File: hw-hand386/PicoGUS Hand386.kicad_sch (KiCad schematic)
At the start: 37 parts, among them J1 AudioJack3, J3 Bus_ISA_8bit, J5 AudioJack3, J6 UART_TX, U1 Pico, U2 SN74CB3T3245, U3 SN74CB3T3257, U4 SN74CB3T3257, U5 74AHC14, U6 74LVC00, U7 74LVC1G00, U8 APS6404L-3SQN-SN, U9 74LVC1G06

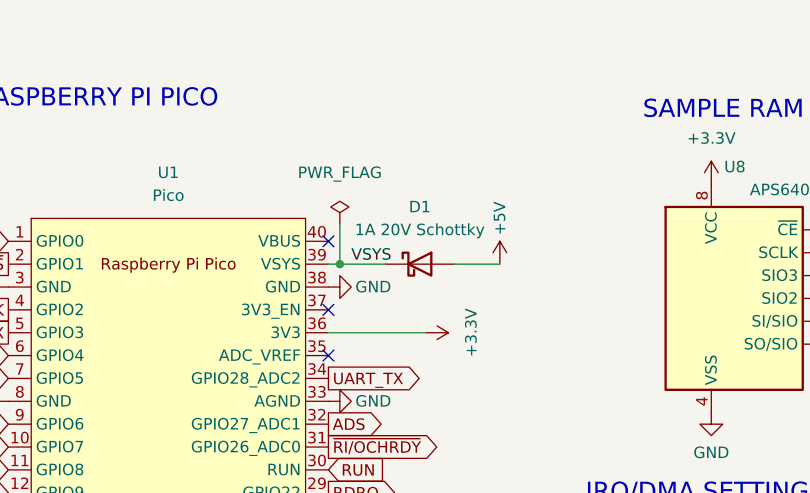
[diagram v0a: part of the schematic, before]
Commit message: v1.3 of Femto edition submitted to JLCPCB 2022-09-26
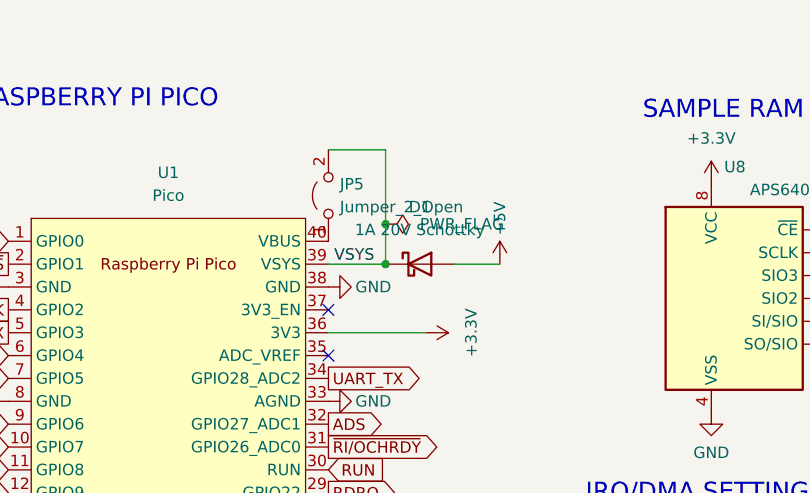
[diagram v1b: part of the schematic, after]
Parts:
- added JP5: Jumper_2_Open, Connector_PinHeader_2.54mm:PinHeader_1x02_P2.54mm_Vertical, symbol Jumper:Jumper_2_Open
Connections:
- net VSYS: now also JP5.2 (B)
- net at U1.40 (VBUS): now also JP5.1 (A)
- no-connect marks 6 -> 5
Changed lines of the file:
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@@
   (junction (at 62.865 182.88) (diameter 0) (color 0 0 0 0)
   )
+  (junction (at 133.35 40.005) (diameter 0) (color 0 0 0 0)
+  )
   (junction (at 217.805 160.655) (diameter 0) (color 0 0 0 0)
   )
@@
   (junction (at 89.535 166.37) (diameter 0) (color 0 0 0 0)
   )
-  (junction (at 128.27 40.005) (diameter 0) (color 0 0 0 0)
-  )
   (junction (at 233.68 153.035) (diameter 0) (color 0 0 0 0)
   )
@@
   )
   (junction (at 47.625 190.5) (diameter 0) (color 0 0 0 0)
+  )
+  (junction (at 133.35 35.56) (diameter 0) (color 0 0 0 0)
   )
   (junction (at 67.945 190.5) (diameter 0) (color 0 0 0 0)
@@
   (no_connect (at 145.415 121.285))
   (no_connect (at 127 50.165))
-  (no_connect (at 127 37.465))
   (no_connect (at 127 45.085))
   (no_connect (at 145.415 136.525))
@@
     (stroke (width 0) (type default))
   )
-  (wire (pts (xy 128.27 40.005) (xy 127 40.005))
+  (wire (pts (xy 127 40.005) (xy 133.35 40.005))
     (stroke (width 0) (type default))
   )
@@
     (stroke (width 0) (type default))
   )
-  (wire (pts (xy 128.27 35.56) (xy 128.27 40.005))
+  (wire (pts (xy 133.35 27.305) (xy 133.35 35.56))
     (stroke (width 0) (type default))
   )
@@
     (stroke (width 0) (type default))
   )
+  (wire (pts (xy 133.35 27.305) (xy 127 27.305))
+    (stroke (width 0) (type default))
+  )
   (wire (pts (xy 175.26 88.265) (xy 175.26 93.345))
     (stroke (width 0) (type default))
@@
     (stroke (width 0) (type default))
   )
-  (wire (pts (xy 133.35 40.005) (xy 128.27 40.005))
-    (stroke (width 0) (type default))
-  )
   (wire (pts (xy 21.59 100.33) (xy 28.575 100.33))
     (stroke (width 0) (type default))
@@
   )
   (wire (pts (xy 180.34 129.54) (xy 189.23 129.54))
+    (stroke (width 0) (type default))
+  )
+  (wire (pts (xy 133.35 35.56) (xy 133.35 40.005))
     (stroke (width 0) (type default))
   )
@@
     (effects (font (size 2 2)) (justify left bottom))
   )
-  (label "VSYS" (at 129.54 40.005 0) (fields_autoplaced)
+  (label "VSYS" (at 127.635 40.005 0) (fields_autoplaced)
     (effects (font (size 1.27 1.27)) (justify left bottom))
   )
@@
     )
   )
+  (symbol (lib_id "Jumper:Jumper_2_Open") (at 127 32.385 90) (unit 1)
+    (in_bom yes) (on_board yes) (dnp no)
+    (property "Reference" "JP5" (at 128.27 31.115 90)
+      (effects (font (size 1.27 1.27)) (justify right))
+    )
+    (property "Value" "Jumper_2_Open" (at 128.27 33.655 90)
+      (effects (font (size 1.27 1.27)) (justify right))
+    )
+    (property "Footprint" "Connector_PinHeader_2.54mm:PinHeader_1x02_P2.54mm_Vertical" (at 127 32.385 0)
+      (effects (font (size 1.27 1.27)) hide)
+    )
+    (property "Datasheet" "~" (at 127 32.385 0)
+      (effects (font (size 1.27 1.27)) hide)
+    )
+    (pin "1")
+    (pin "2")
+    (instances
+      (project "PicoGUS Hand386"
+        (path "/8fb4b197-630e-4faa-9892-8ecaeb71c13b"
+          (reference "JP5") (unit 1)
+        )
+      )
+    )
+  )
   (symbol (lib_id "Device:D_Schottky") (at 137.16 40.005 0) (unit 1)
     (in_bom yes) (on_board yes) (dnp no)
@@
     )
   )
-  (symbol (lib_id "power:PWR_FLAG") (at 128.27 35.56 0) (unit 1)
+  (symbol (lib_id "power:PWR_FLAG") (at 133.35 35.56 270) (unit 1)
     (in_bom yes) (on_board yes) (dnp no) (fields_autoplaced)
-    (property "Reference" "#FLG0101" (at 128.27 33.655 0)
-      (effects (font (size 1.27 1.27)) hide)
-    )
-    (property "Value" "PWR_FLAG" (at 128.27 29.845 0)
-      (effects (font (size 1.27 1.27)))
-    )
-    (property "Footprint" "" (at 128.27 35.56 0)
-      (effects (font (size 1.27 1.27)) hide)
-    )
-    (property "Datasheet" "~" (at 128.27 35.56 0)
-      (effects (font (size 1.27 1.27)) hide)
-    )
+    (property "Reference" "#FLG0101" (at 135.255 35.56 0)
+      (effects (font (size 1.27 1.27)) hide)
+    )
+    (property "Value" "PWR_FLAG" (at 137.16 35.56 90)
+      (effects (font (size 1.27 1.27)) (justify left))
+    )
+    (property "Footprint" "" (at 133.35 35.56 0)
+      (effects (font (size 1.27 1.27)) hide)
+    )
+    (property "Datasheet" "~" (at 133.35 35.56 0)
+      (effects (font (size 1.27 1.27)) hide)
+    )
